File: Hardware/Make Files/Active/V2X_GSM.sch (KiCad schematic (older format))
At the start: 46 parts, among them P1 47553-1001, P14 CUR_SEN, P2 SMA, P26 CONN_02X08, P3 SMA, Q12 IRF9335, U13 XRP6124, U3 MMQA5V6T3G, U4 SIM5320

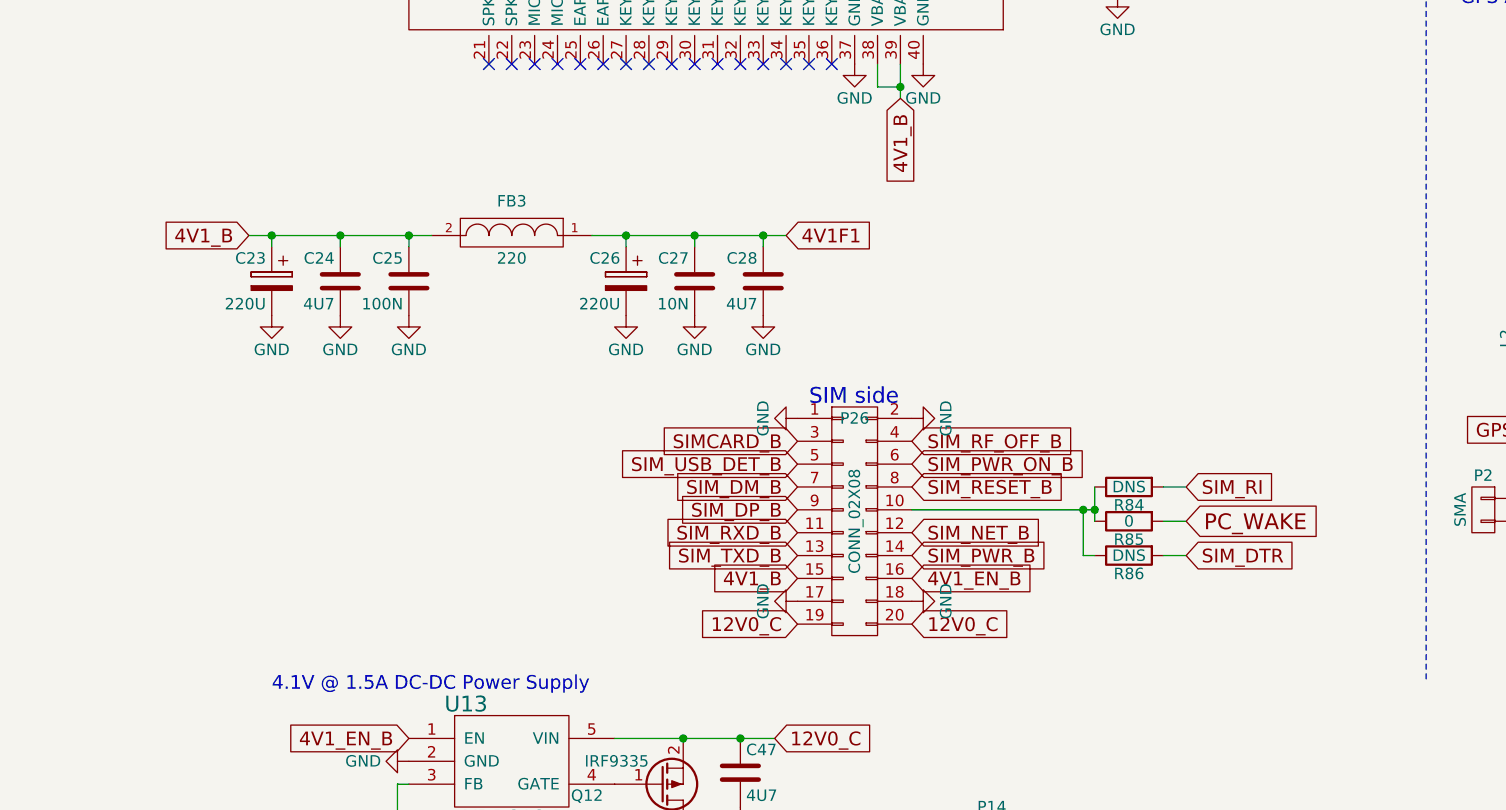
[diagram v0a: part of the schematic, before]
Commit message: work from home day
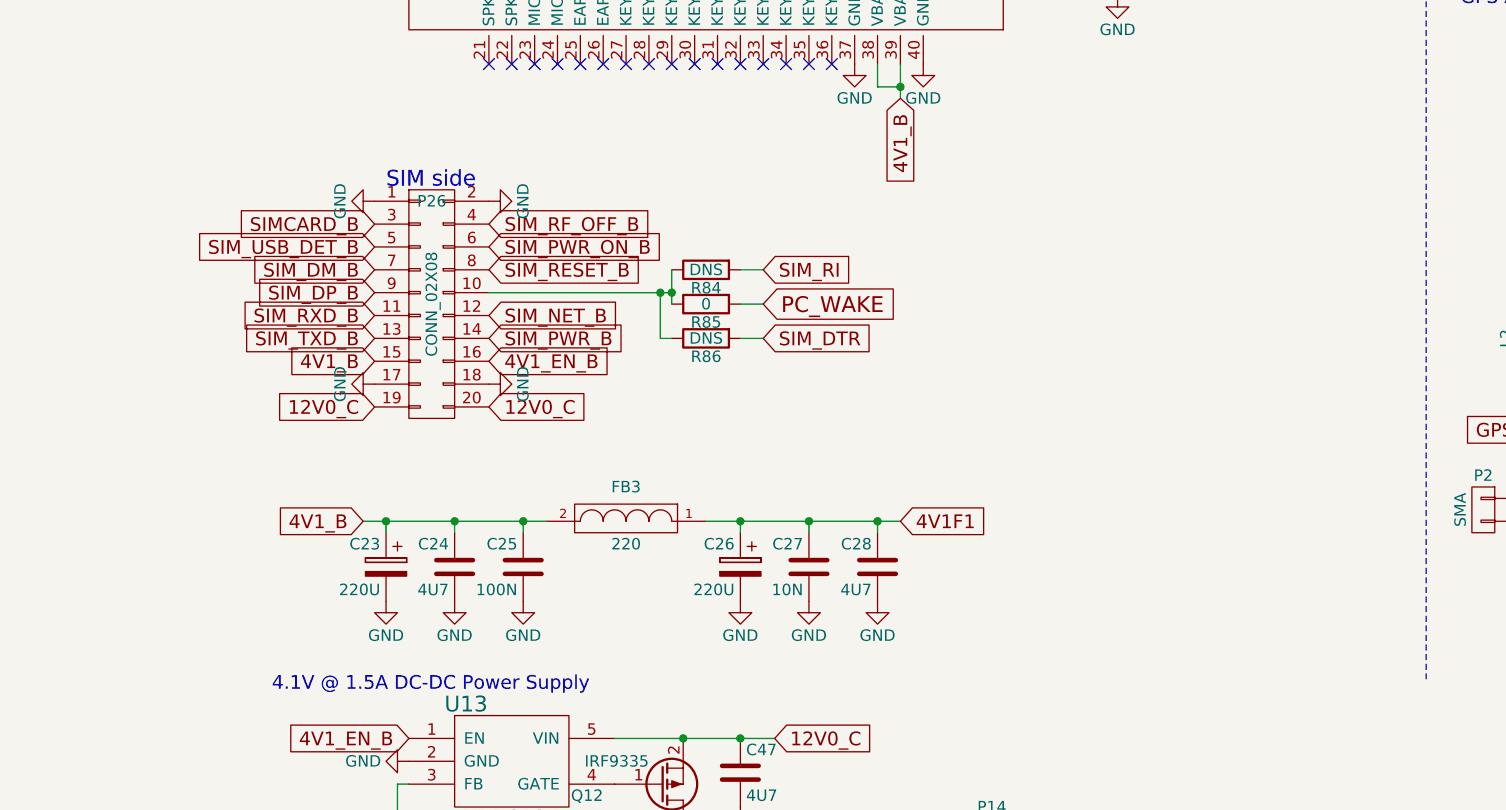
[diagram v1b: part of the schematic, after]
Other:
- moved on the sheet: C23, C24, C25, C26, C27, C28, FB3, P26, R84, R85, R86
